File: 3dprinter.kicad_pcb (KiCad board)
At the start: 2 copper layers, 125.2 x 75.2 mm, 86 parts, among them J1 6P IDC CONNECTOR, J10 X, J11 E, J12 YM, J13 Y, J14 ZM, J15 Z, J16 Z, J17 Conn_01x02, J2 USB_B, J3 X-, J4 Thermistor, J5 Y-, J6 Z-, J7 Heaters & Fans, J8 XM, J9 EM, SW1 SW_Push, U1 ATmega2560-16A, U2 CH340G, U3 LM78M05_TO252, Y1 16MHZ, Y2 12MHZ

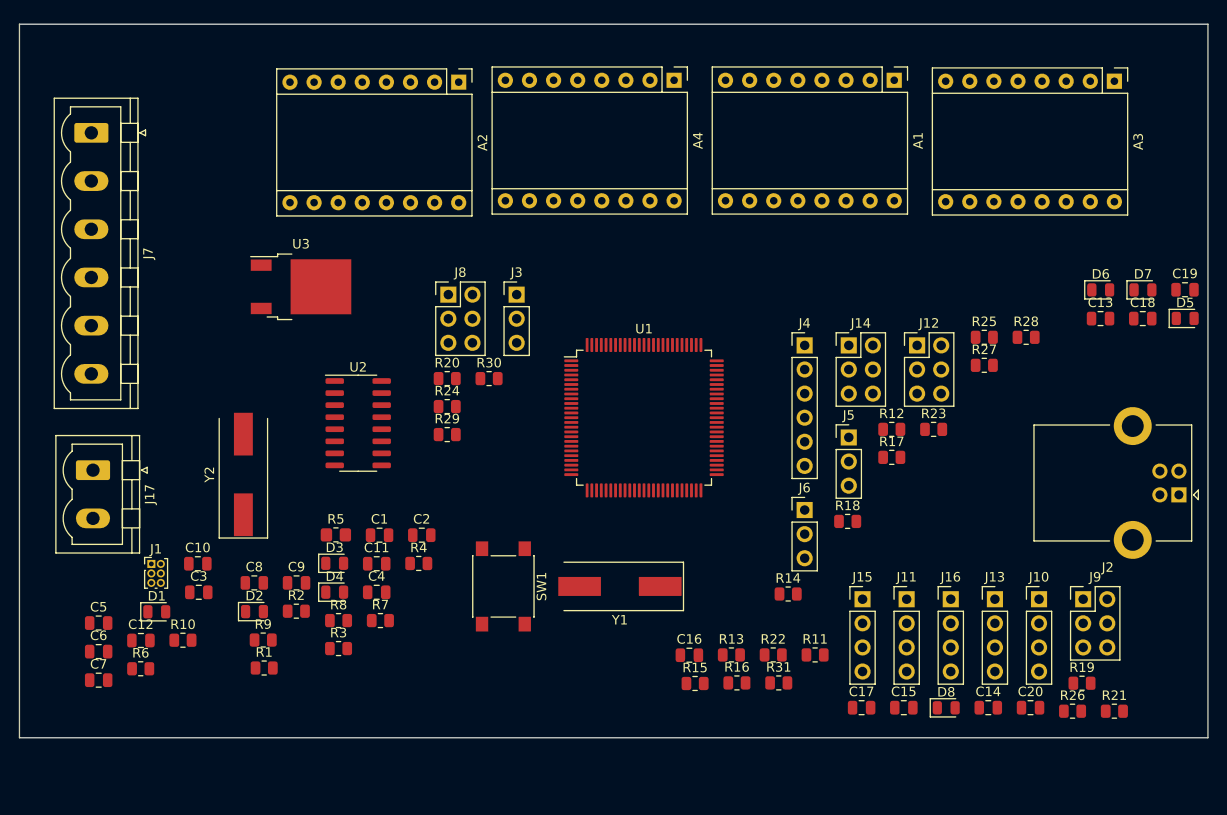
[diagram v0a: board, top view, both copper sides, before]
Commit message: hebele
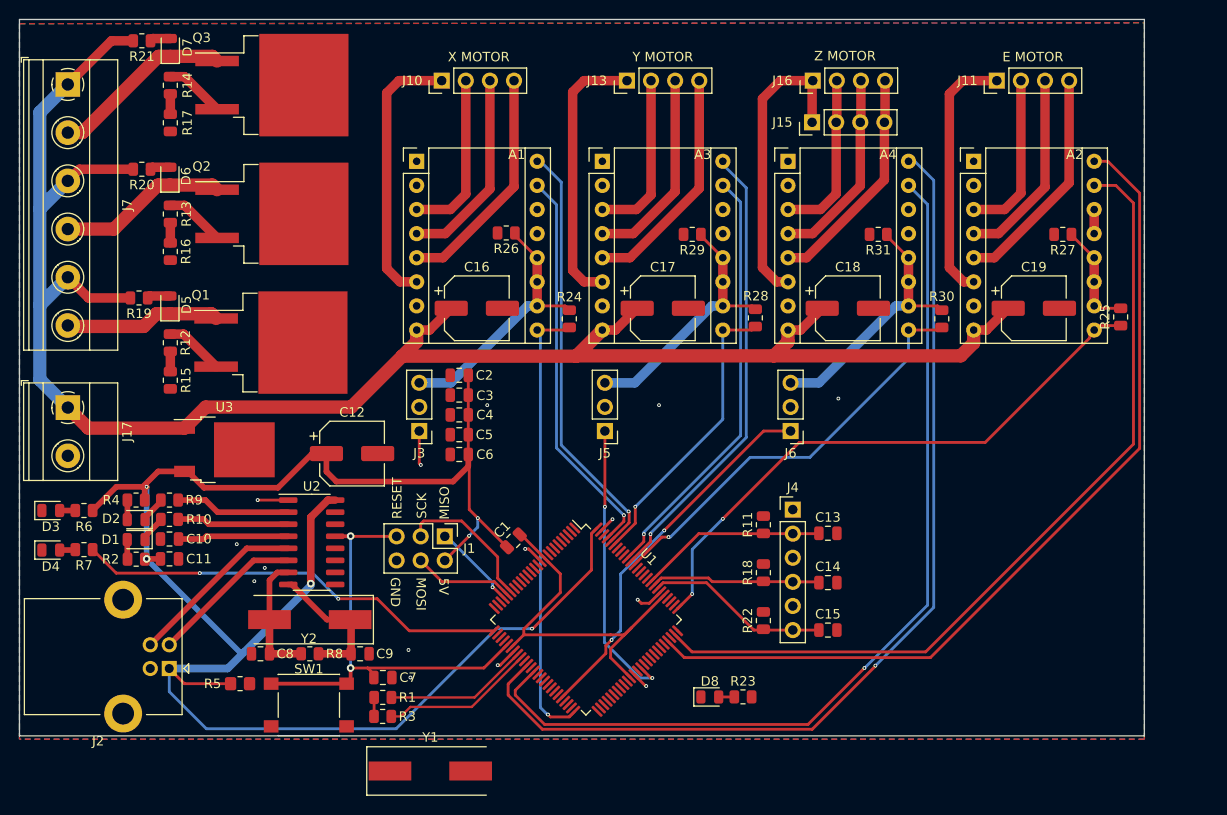
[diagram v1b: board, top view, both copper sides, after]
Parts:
- removed C20: 100uF, Capacitor_SMD:C_0805_2012Metric
- removed J12: YM, Connector_PinHeader_2.54mm:PinHeader_2x03_P2.54mm_Vertical
- removed J14: ZM, Connector_PinHeader_2.54mm:PinHeader_2x03_P2.54mm_Vertical
- removed J8: XM, Connector_PinHeader_2.54mm:PinHeader_2x03_P2.54mm_Vertical
- removed J9: EM, Connector_PinHeader_2.54mm:PinHeader_2x03_P2.54mm_Vertical
- added Q1: Mos, Package_TO_SOT_SMD:TO-263-2, F.Cu at (120.7, 101.3)
- added Q2: Mos, Package_TO_SOT_SMD:TO-263-2, F.Cu at (120.8, 87.7)
- added Q3: Mos, Package_TO_SOT_SMD:TO-263-2, F.Cu at (120.8, 74.2)
- C12, C16, C17, C18, C19: footprint Capacitor_SMD:C_0805_2012Metric -> Capacitor_SMD:CP_Elec_6.3x7.7
- J1: footprint Connector_PinHeader_1.00mm:PinHeader_2x03_P1.00mm_Vertical -> Connector_PinHeader_2.54mm:PinHeader_2x03_P2.54mm_Vertical
- J17: footprint Connector_Phoenix_MSTB:PhoenixContact_MSTBVA_2,5_2-G-5,08_1x02_P5.08mm_Vertical -> TerminalBlock_Phoenix:TerminalBlock_Phoenix_MKDS-1,5-2-5.08_1x02_P5.08mm_Horizontal
- J7: footprint Connector_Phoenix_MSTB:PhoenixContact_MSTBVA_2,5_6-G-5,08_1x06_P5.08mm_Vertical -> TerminalBlock_Phoenix:TerminalBlock_Phoenix_MKDS-1,5-6-5.08_1x06_P5.08mm_Horizontal
- moved R21 124.5 mm to (107.1, 69.5), turned to 180 degrees
- moved J2 108.0 mm to (110.0, 135.7)
- moved R19 107.4 mm to (106.8, 96.6), turned to 180 degrees
- moved D5 107.0 mm to (110.1, 97.3), turned to 90 degrees
- moved D7 105.6 mm to (110.1, 70.2), turned to 90 degrees
- moved D6 98.8 mm to (110.1, 83.8), turned to 90 degrees
- moved R14 84.3 mm to (110.1, 74.2), turned to 90 degrees
- moved R17 83.8 mm to (110.1, 78.1), turned to -90 degrees
- moved J10 83.4 mm to (138.7, 73.7), turned to 90 degrees
- moved R26 78.1 mm to (145.5, 89.8), turned to 180 degrees
- moved R12 76.6 mm to (110.1, 101.3), turned to 90 degrees
- moved R13 75.2 mm to (110.1, 87.8), turned to 90 degrees
- moved R16 75.0 mm to (110.1, 91.7), turned to -90 degrees
- moved J13 67.0 mm to (158.2, 73.7), turned to 90 degrees
- moved R15 63.9 mm to (110.1, 105.3), turned to -90 degrees
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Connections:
- A1 pad 10: MX0 -> ME0
- A1 pad 11: MX1 -> ME0
- A1 pad 12: MX2 -> ME0
- A2 pad 11: ME1 -> ME0
- A2 pad 12: ME2 -> ME0
- A3 pad 10: MY0 -> ME0
- A3 pad 11: MY1 -> ME0
- A3 pad 12: MY2 -> ME0
- A4 pad 10: MZ0 -> ME0
- A4 pad 11: MZ1 -> ME0
- A4 pad 12: MZ2 -> ME0
- J1 pad 1: PB3(MISO) -> MISO
- J1 pad 3: PB1(SCK) -> SCK
- J1 pad 4: PB2(MOSI) -> MOSI
- J3 pad 3: 5V -> ME0
- J5 pad 3: 5V -> ME0
- J6 pad 3: 5V -> ME0
- R11 pad 2: 5V -> ME0
- R18 pad 2: 5V -> ME0
- R22 pad 2: 5V -> ME0
- R24 pad 2: 5V -> ME0
- R25 pad 2: 5V -> ME0
- R26 pad 1: MX0 -> ME0
- R28 pad 2: 5V -> ME0
- R29 pad 1: MY0 -> ME0
- R30 pad 2: 5V -> ME0
- R31 pad 1: MZ0 -> ME0
- U1 pad 26: unconnected-(U1-Pad26) -> PB7
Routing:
- net 12V: track 0.00 -> 198.9 mm
- net 5V: track 0.00 -> 195.1 mm, vias 0 -> 6
- net ZDIR: track 0.00 -> 104.3 mm, vias 0 -> 1
- net ZSTEP: track 0.00 -> 98.4 mm, vias 0 -> 1
- net ME0: track 0.00 -> 95.3 mm
- net EDIR: track 0.00 -> 92.7 mm
- net ESTEP: track 0.00 -> 88.5 mm
- net E0-EN: track 0.00 -> 62.0 mm, vias 0 -> 2
- net RESET: track 0.00 -> 49.0 mm, vias 0 -> 2
- net YDIR: track 0.00 -> 48.2 mm, vias 0 -> 1
- net X-EN: track 0.00 -> 47.7 mm, vias 0 -> 1
- net PB7: track 0.00 -> 45.9 mm, vias 0 -> 2
- net XDIR: track 0.00 -> 45.1 mm, vias 0 -> 1
- net YSTEP: track 0.00 -> 45.1 mm, vias 0 -> 1
- net Z-EN: track 0.00 -> 44.6 mm, vias 0 -> 1
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- added copper zone on B.Cu, net GND
- added copper zone on F.Cu, net GND
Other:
- board size 125.2 x 75.2 mm -> 118.5 x 75.5 mm
- board text added: "5V"
- board text added: "E MOTOR"
- board text added: "GND"
- board text added: "MISO"
- board text added: "MOSI"
- board text added: "RESET"
- board text added: "SCK"
- board text added: "X MOTOR"
- board text added: "Y MOTOR"
- board text added: "Z MOTOR"

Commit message: Schematic_ok
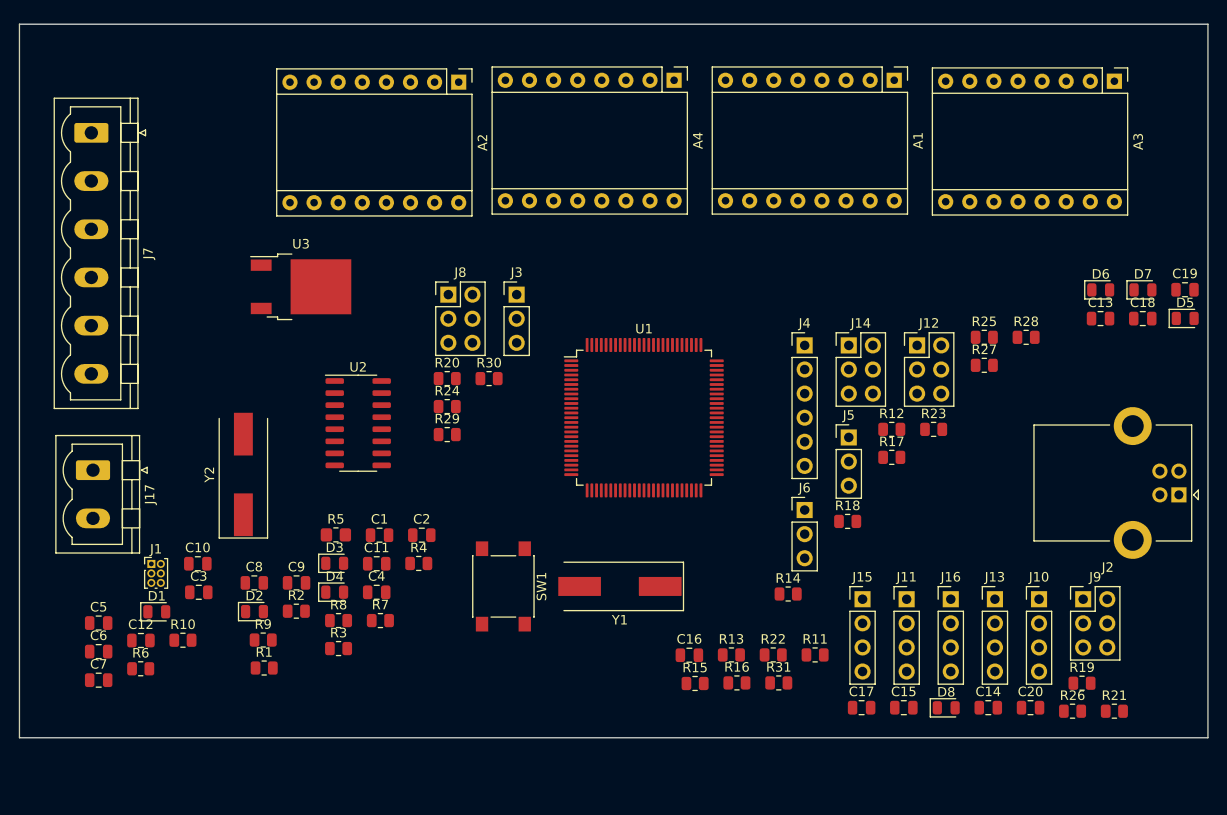
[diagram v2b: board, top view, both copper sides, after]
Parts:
- removed Q1, Q2, Q3: Mos, Package_TO_SOT_SMD:TO-263-2
- added C20: 100uF, Capacitor_SMD:C_0805_2012Metric, F.Cu at (200.8, 139.8)
- added J12: YM, Connector_PinHeader_2.54mm:PinHeader_2x03_P2.54mm_Vertical, F.Cu at (188.8, 101.6)
- added J14: ZM, Connector_PinHeader_2.54mm:PinHeader_2x03_P2.54mm_Vertical, F.Cu at (181.6, 101.6)
- added J8: XM, Connector_PinHeader_2.54mm:PinHeader_2x03_P2.54mm_Vertical, F.Cu at (139.4, 96.2)
- added J9: EM, Connector_PinHeader_2.54mm:PinHeader_2x03_P2.54mm_Vertical, F.Cu at (206.3, 128.3)
- C12, C16, C17, C18, C19: footprint Capacitor_SMD:CP_Elec_6.3x7.7 -> Capacitor_SMD:C_0805_2012Metric
- J1: footprint Connector_PinHeader_2.54mm:PinHeader_2x03_P2.54mm_Vertical -> Connector_PinHeader_1.00mm:PinHeader_2x03_P1.00mm_Vertical
- J17: footprint TerminalBlock_Phoenix:TerminalBlock_Phoenix_MKDS-1,5-2-5.08_1x02_P5.08mm_Horizontal -> Connector_Phoenix_MSTB:PhoenixContact_MSTBVA_2,5_2-G-5,08_1x02_P5.08mm_Vertical
- J7: footprint TerminalBlock_Phoenix:TerminalBlock_Phoenix_MKDS-1,5-6-5.08_1x06_P5.08mm_Horizontal -> Connector_Phoenix_MSTB:PhoenixContact_MSTBVA_2,5_6-G-5,08_1x06_P5.08mm_Vertical
- moved R21 124.5 mm to (209.6, 140.2), turned to 0 degrees
- moved J2 108.0 mm to (216.4, 117.3)
- moved R19 107.4 mm to (206.2, 137.2), turned to 0 degrees
- moved D5 107.0 mm to (217.1, 98.8), turned to 0 degrees
- moved D7 105.6 mm to (212.6, 95.8), turned to 0 degrees
- moved D6 98.8 mm to (208.2, 95.8), turned to 0 degrees
- moved R14 84.3 mm to (175.2, 127.8), turned to 0 degrees
- moved R17 83.8 mm to (186.1, 113.4), turned to 0 degrees
- moved J10 83.4 mm to (201.7, 128.3), turned to 0 degrees
- moved R26 78.1 mm to (205.2, 140.2), turned to 0 degrees
- moved R12 76.6 mm to (186.1, 110.5), turned to 0 degrees
- moved R13 75.2 mm to (169.2, 134.2), turned to 0 degrees
- moved R16 75.0 mm to (169.8, 137.2), turned to 0 degrees
- moved J13 67.0 mm to (197.0, 128.3), turned to 0 degrees
- moved R15 63.9 mm to (165.4, 137.2), turned to 0 degrees
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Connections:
- A1 pad 10: ME0 -> MX0
- A1 pad 11: ME0 -> MX1
- A1 pad 12: ME0 -> MX2
- A2 pad 11: ME0 -> ME1
- A2 pad 12: ME0 -> ME2
- A3 pad 10: ME0 -> MY0
- A3 pad 11: ME0 -> MY1
- A3 pad 12: ME0 -> MY2
- A4 pad 10: ME0 -> MZ0
- A4 pad 11: ME0 -> MZ1
- A4 pad 12: ME0 -> MZ2
- J1 pad 1: MISO -> PB3(MISO)
- J1 pad 3: SCK -> PB1(SCK)
- J1 pad 4: MOSI -> PB2(MOSI)
- J3 pad 3: ME0 -> 5V
- J5 pad 3: ME0 -> 5V
- J6 pad 3: ME0 -> 5V
- R11 pad 2: ME0 -> 5V
- R18 pad 2: ME0 -> 5V
- R22 pad 2: ME0 -> 5V
- R24 pad 2: ME0 -> 5V
- R25 pad 2: ME0 -> 5V
- R26 pad 1: ME0 -> MX0
- R28 pad 2: ME0 -> 5V
- R29 pad 1: ME0 -> MY0
- R30 pad 2: ME0 -> 5V
- R31 pad 1: ME0 -> MZ0
- U1 pad 26: PB7 -> unconnected-(U1-Pad26)
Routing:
- net 12V: track 198.9 -> 0.00 mm
- net 5V: track 195.1 -> 0.00 mm, vias 6 -> 0
- net ZDIR: track 104.3 -> 0.00 mm, vias 1 -> 0
- net ZSTEP: track 98.4 -> 0.00 mm, vias 1 -> 0
- net ME0: track 95.3 -> 0.00 mm
- net EDIR: track 92.7 -> 0.00 mm
- net ESTEP: track 88.5 -> 0.00 mm
- net E0-EN: track 62.0 -> 0.00 mm, vias 2 -> 0
- net RESET: track 49.0 -> 0.00 mm, vias 2 -> 0
- net YDIR: track 48.2 -> 0.00 mm, vias 1 -> 0
- net X-EN: track 47.7 -> 0.00 mm, vias 1 -> 0
- net PB7: track 45.9 -> 0.00 mm, vias 2 -> 0
- net XDIR: track 45.1 -> 0.00 mm, vias 1 -> 0
- net YSTEP: track 45.1 -> 0.00 mm, vias 1 -> 0
- net Z-EN: track 44.6 -> 0.00 mm, vias 1 -> 0
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- removed copper zone on B.Cu, net GND
- removed copper zone on F.Cu, net GND
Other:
- board size 118.5 x 75.5 mm -> 125.2 x 75.2 mm
- board text removed: "5V"
- board text removed: "E MOTOR"
- board text removed: "GND"
- board text removed: "MISO"
- board text removed: "MOSI"
- board text removed: "RESET"
- board text removed: "SCK"
- board text removed: "X MOTOR"
- board text removed: "Y MOTOR"
- board text removed: "Z MOTOR"
